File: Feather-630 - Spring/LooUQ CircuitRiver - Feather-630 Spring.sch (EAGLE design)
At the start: 23 parts, among them J1 FEATHERHOST-S, J2 FEATHERHOST-L, J3 CR-SPRING_HEADER, J4 JST_PH-2_T/H, J5 JST_PH-2_T/H, J6 QWIIC_VERTICAL, J7 CR-RAPIDSIO_VERTICAL, J8 DNF, P3 SLEEP, U2 LM2674_BUCK

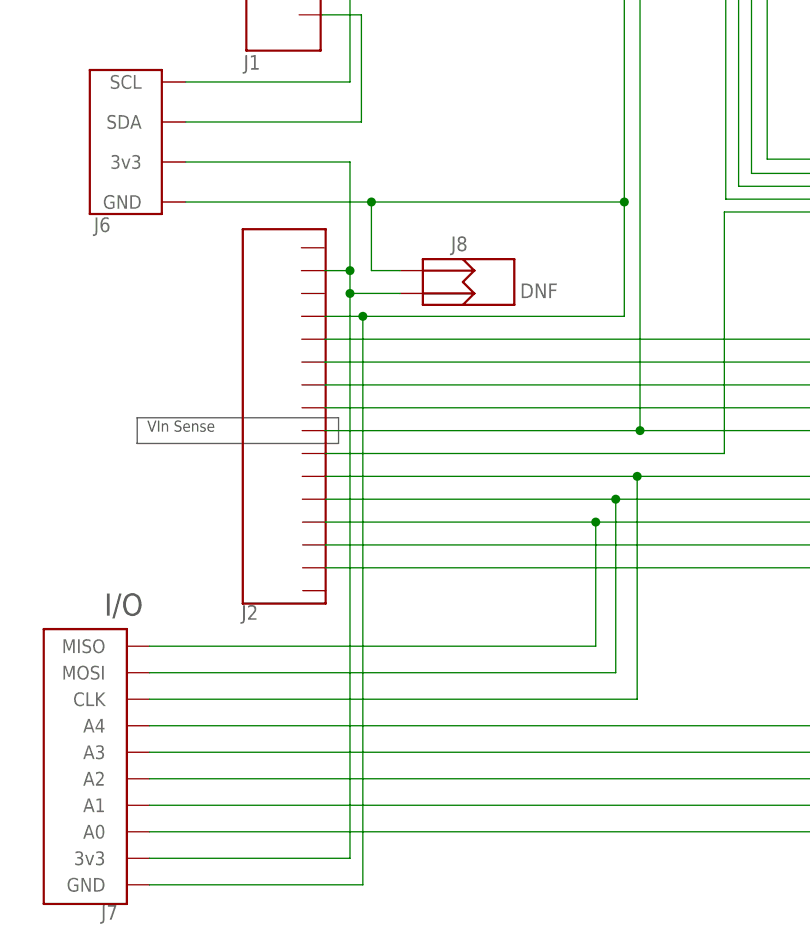
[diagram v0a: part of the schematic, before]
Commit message: Updated Feathers
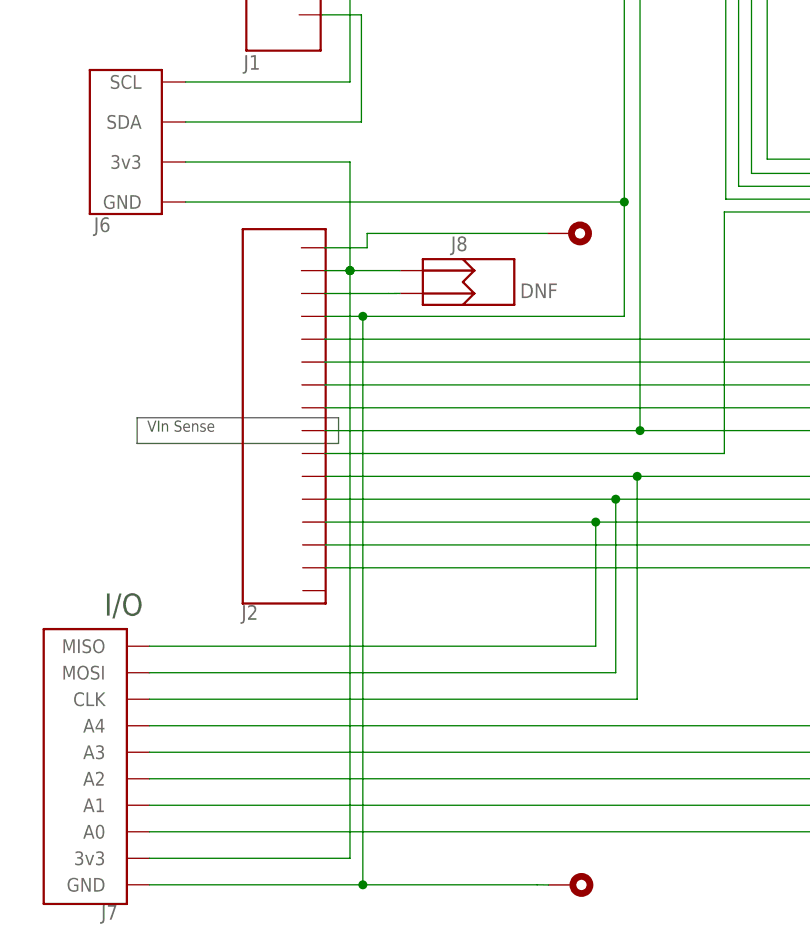
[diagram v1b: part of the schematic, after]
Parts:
- added P1, P2: DNF, common:DNF
- P3: value SLEEP -> DNF; device common:SLEEP -> common:DNF
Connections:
- new net Net_29: J2.AREF, J8.P1
- new net Net_30: J2.!RESET, P1.1
- net Net_3v3: now also J8.P2; no longer J8.P1
- net Net_GND: now also P2.1; no longer J8.P2
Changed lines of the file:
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@@
 <part name="LG1" library="common" deviceset="LOOUQ_LOGO" device=""/>
 <part name="LG2" library="common" deviceset="CIRCUITRIVER_LOGO" device=""/>
-<part name="P3" library="common" deviceset="SLEEP" device=""/>
+<part name="P1" library="common" deviceset="DNF" device=""/>
+<part name="P2" library="common" deviceset="DNF" device=""/>
+<part name="P3" library="common" deviceset="DNF" device=""/>
 <part name="R1" library="common" deviceset="RES_0603" device="" value="12M"/>
 <part name="R2" library="common" deviceset="RES_0603" device="" value="1.5M"/>
@@
 <instance part="LG1" gate="PART_1" x="114.776" y="131.128"/>
 <instance part="LG2" gate="PART_1" x="115.24" y="125.093"/>
+<instance part="P1" gate="BRKOUTPAD" x="-57.229" y="-13.176" rot="R90"/>
+<instance part="P2" gate="BRKOUTPAD" x="-57.071" y="-85.566" rot="R90"/>
 <instance part="P3" gate="BRKOUTPAD" x="101.362" y="-6.033" rot="R270"/>
 <instance part="R1" gate="PART_1" x="-52.223" y="100.477" rot="R90">
@@
 <busses/>
 <nets>
-<net name="Net_VBUS" class="1">
-<segment>
-<wire layer="91" width="0.25" x1="73.028" y1="78.581" x2="73.028" y2="51.594"/>
-<wire layer="91" width="0.25" x1="73.028" y1="51.594" x2="-61.913" y2="51.594"/>
-<wire layer="91" width="0.25" x1="-61.913" y1="51.594" x2="-61.913" y2="33.969"/>
-<wire layer="91" width="0.25" x1="-61.913" y1="33.969" x2="-85.94" y2="33.969"/>
-<pinref part="D2" gate="PART_1" pin="C"/>
-<pinref part="J1" gate="PART_1" pin="VBUS"/>
-</segment>
-</net>
 <net name="Net_1" class="0">
 <segment>
@@
 <pinref part="J7" gate="PART_1" pin="MISO"/>
 <junction x="-55.404" y="-45.248"/>
-</segment>
-</net>
-<net name="Net_VSW" class="1">
-<segment>
-<wire layer="91" width="0.25" x1="32.861" y1="88.741" x2="32.861" y2="101.113"/>
-<wire layer="91" width="0.25" x1="32.861" y1="101.113" x2="36.189" y2="101.113"/>
-<pinref part="D1" gate="PART_1" pin="C"/>
-<pinref part="L1" gate="PART_1" pin="1"/>
-<wire layer="91" width="0.25" x1="-5.106" y1="111.81" x2="-3.836" y2="111.81"/>
-<wire layer="91" width="0.25" x1="-5.106" y1="111.81" x2="-5.106" y2="101.113"/>
-<wire layer="91" width="0.25" x1="-5.106" y1="101.113" x2="32.861" y2="101.113"/>
-<pinref part="U2" gate="PART_1" pin="VSW"/>
-<junction x="32.861" y="101.113"/>
-<wire layer="91" width="0.25" x1="30.318" y1="111.748" x2="32.861" y2="111.748"/>
-<wire layer="91" width="0.25" x1="32.861" y1="111.748" x2="32.861" y2="101.113"/>
-<pinref part="C3" gate="PART_1" pin="2"/>
-<junction x="32.861" y="101.113"/>
 </segment>
 </net>
@@
 </segment>
 </net>
+<net name="Net_29" class="0">
+<segment>
+<wire layer="91" width="0.25" x1="-78.423" y1="-19.848" x2="-77.153" y2="-19.844"/>
+<wire layer="91" width="0.25" x1="-78.423" y1="-19.848" x2="-85.552" y2="-19.848"/>
+<pinref part="J8" gate="PART_1" pin="P1"/>
+<pinref part="J2" gate="PART_1" pin="AREF"/>
+</segment>
+</net>
+<net name="Net_30" class="0">
+<segment>
+<wire layer="91" width="0.25" x1="-60.801" y1="-13.176" x2="-80.804" y2="-13.176"/>
+<wire layer="91" width="0.25" x1="-80.804" y1="-13.176" x2="-80.804" y2="-14.768"/>
+<wire layer="91" width="0.25" x1="-80.804" y1="-14.768" x2="-85.573" y2="-14.768"/>
+<pinref part="P1" gate="BRKOUTPAD" pin="1"/>
+<pinref part="J2" gate="PART_1" pin="!RESET"/>
+</segment>
+</net>
 <net name="Net_3v3" class="1">
 <segment>
-<wire layer="91" width="0.25" x1="-77.153" y1="-19.844" x2="-82.709" y2="-19.844"/>
-<wire layer="91" width="0.25" x1="-82.709" y1="-19.844" x2="-82.709" y2="-17.308"/>
+<wire layer="91" width="0.25" x1="-100.965" y1="-5.239" x2="-82.709" y2="-5.239"/>
+<wire layer="91" width="0.25" x1="-82.709" y1="-17.304" x2="-82.709" y2="-17.308"/>
+<wire layer="91" width="0.25" x1="-82.709" y1="-5.239" x2="-82.709" y2="-17.304"/>
 <wire layer="91" width="0.25" x1="-82.709" y1="-17.308" x2="-85.563" y2="-17.308"/>
-<pinref part="J8" gate="PART_1" pin="P1"/>
+<pinref part="J6" gate="PART_1" pin="3v3"/>
 <pinref part="J2" gate="PART_1" pin="+3V3"/>
-<wire layer="91" width="0.25" x1="-100.965" y1="-5.239" x2="-82.709" y2="-5.239"/>
-<wire layer="91" width="0.25" x1="-82.709" y1="-5.239" x2="-82.709" y2="-17.308"/>
-<pinref part="J6" gate="PART_1" pin="3v3"/>
-<junction x="-82.709" y="-17.308"/>
-<wire layer="91" width="0.25" x1="-82.709" y1="-19.844" x2="-82.709" y2="-82.605"/>
+<wire layer="91" width="0.25" x1="-82.709" y1="-17.308" x2="-82.709" y2="-82.605"/>
 <wire layer="91" width="0.25" x1="-82.709" y1="-82.605" x2="-104.989" y2="-82.605"/>
 <pinref part="J7" gate="PART_1" pin="3v3"/>
-<junction x="-82.709" y="-19.844"/>
+<junction x="-82.709" y="-17.308"/>
+<wire layer="91" width="0.25" x1="-77.153" y1="-17.304" x2="-82.709" y2="-17.304"/>
+<pinref part="J8" gate="PART_1" pin="P2"/>
+<junction x="-82.709" y="-17.304"/>
 </segment>
 </net>
@@
 <pinref part="J4" gate="PART_1" pin="P2"/>
 <junction x="93.504" y="44.05"/>
-<wire layer="91" width="0.25" x1="-100.965" y1="-9.684" x2="-80.327" y2="-9.684"/>
-<wire layer="91" width="0.25" x1="-80.327" y1="-9.684" x2="-52.229" y2="-9.684"/>
+<wire layer="91" width="0.25" x1="-100.965" y1="-9.684" x2="-52.229" y2="-9.684"/>
 <pinref part="J6" gate="PART_1" pin="GND"/>
 <junction x="-52.229" y="-9.684"/>
-<wire layer="91" width="0.25" x1="-77.153" y1="-17.304" x2="-80.327" y2="-17.304"/>
-<wire layer="91" width="0.25" x1="-80.327" y1="-17.304" x2="-80.327" y2="-9.684"/>
-<pinref part="J8" gate="PART_1" pin="P2"/>
-<junction x="-80.327" y="-9.684"/>
 <wire layer="91" width="0.25" x1="-81.28" y1="-22.388" x2="-81.28" y2="-85.551"/>
 <wire layer="91" width="0.25" x1="-81.28" y1="-85.551" x2="-104.989" y2="-85.551"/>
 <pinref part="J7" gate="PART_1" pin="GND"/>
 <junction x="-81.28" y="-22.388"/>
+<wire layer="91" width="0.25" x1="-61.912" y1="-85.551" x2="-60.643" y2="-85.566"/>
+<wire layer="91" width="0.25" x1="-61.912" y1="-85.551" x2="-81.28" y2="-85.551"/>
+<pinref part="P2" gate="BRKOUTPAD" pin="1"/>
+<junction x="-81.28" y="-85.551"/>
 </segment>
 </net>
@@
 <pinref part="J4" gate="PART_1" pin="P1"/>
 <junction x="97.621" y="39.048"/>
+</segment>
+</net>
+<net name="Net_VBUS" class="1">
+<segment>
+<wire layer="91" width="0.25" x1="73.028" y1="78.581" x2="73.028" y2="51.594"/>
+<wire layer="91" width="0.25" x1="73.028" y1="51.594" x2="-61.913" y2="51.594"/>
+<wire layer="91" width="0.25" x1="-61.913" y1="51.594" x2="-61.913" y2="33.969"/>
+<wire layer="91" width="0.25" x1="-61.913" y1="33.969" x2="-85.94" y2="33.969"/>
+<pinref part="D2" gate="PART_1" pin="C"/>
+<pinref part="J1" gate="PART_1" pin="VBUS"/>
 </segment>
 </net>
@@
 </segment>
 </net>
+<net name="Net_VSW" class="1">
+<segment>
+<wire layer="91" width="0.25" x1="32.861" y1="88.741" x2="32.861" y2="101.113"/>
+<wire layer="91" width="0.25" x1="32.861" y1="101.113" x2="36.189" y2="101.113"/>
+<pinref part="D1" gate="PART_1" pin="C"/>
+<pinref part="L1" gate="PART_1" pin="1"/>
+<wire layer="91" width="0.25" x1="-5.106" y1="111.81" x2="-3.836" y2="111.81"/>
+<wire layer="91" width="0.25" x1="-5.106" y1="111.81" x2="-5.106" y2="101.113"/>
+<wire layer="91" width="0.25" x1="-5.106" y1="101.113" x2="32.861" y2="101.113"/>
+<pinref part="U2" gate="PART_1" pin="VSW"/>
+<junction x="32.861" y="101.113"/>
+<wire layer="91" width="0.25" x1="30.318" y1="111.748" x2="32.861" y2="111.748"/>
+<wire layer="91" width="0.25" x1="32.861" y1="111.748" x2="32.861" y2="101.113"/>
+<pinref part="C3" gate="PART_1" pin="2"/>
+<junction x="32.861" y="101.113"/>
+</segment>
+</net>
